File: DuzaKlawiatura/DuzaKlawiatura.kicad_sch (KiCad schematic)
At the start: 29 parts, among them J1 Conn_01x02_Pin, J2 Conn_01x02_Pin, J3 USB_C_Receptacle_USB2.0, U6 STM32F072CBT6, U7 SN74LV1T34DBV, U8 PRTR5V0U2X, U9 XC6206P332MR-Regulator_Linear

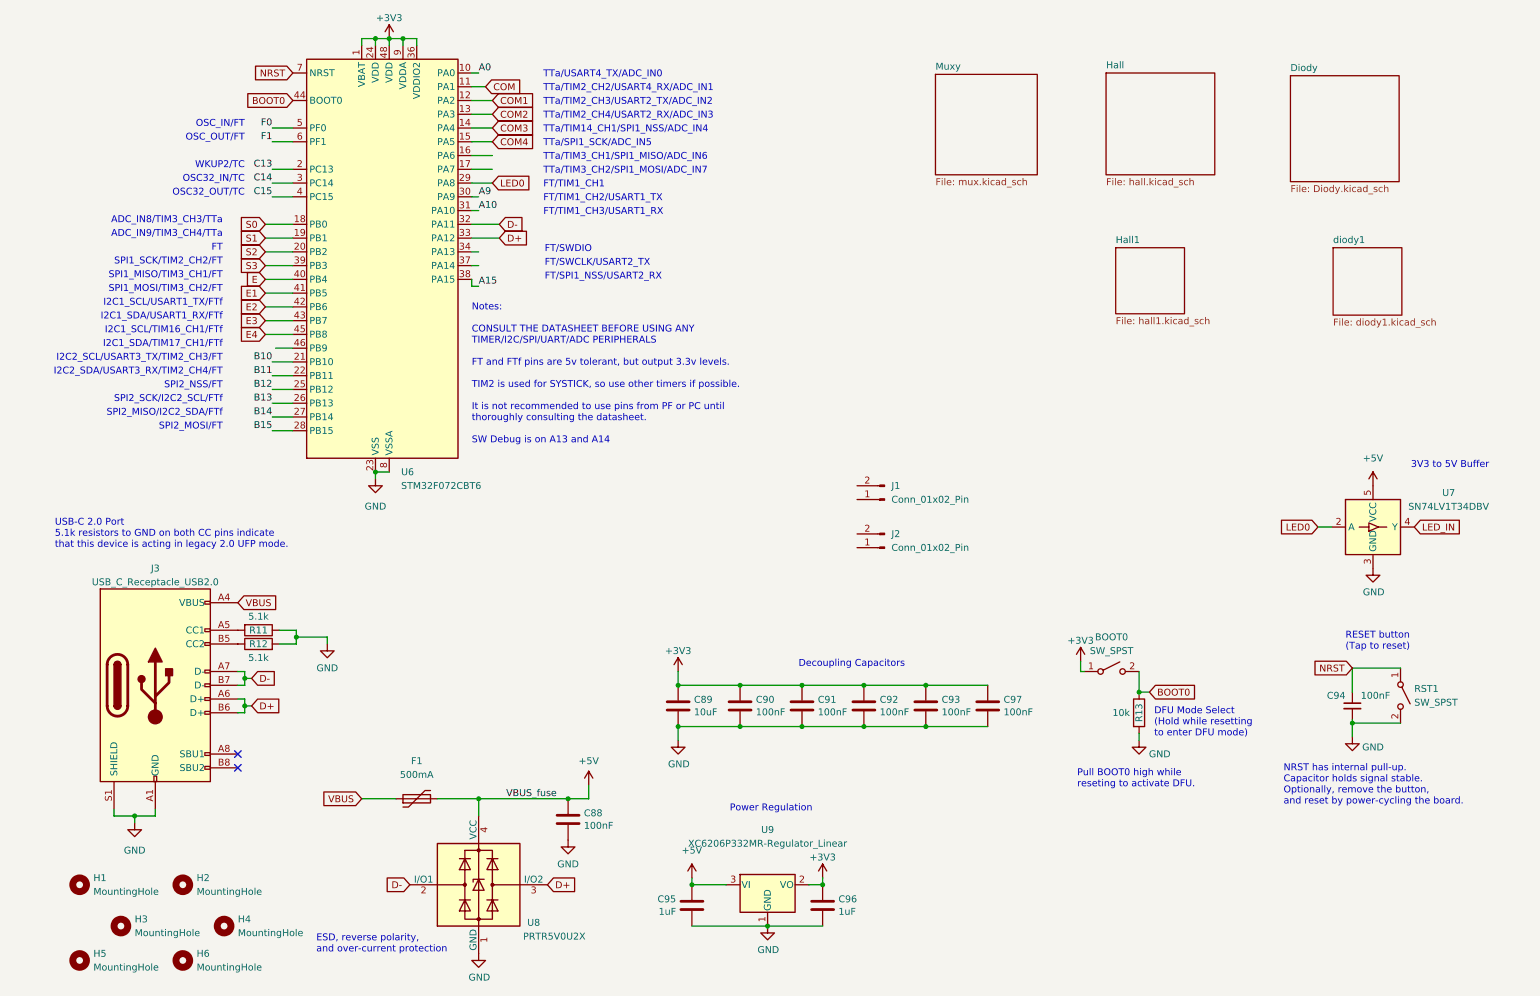
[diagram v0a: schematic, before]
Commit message: Added photos of layout and schematic, updated Kicad files.
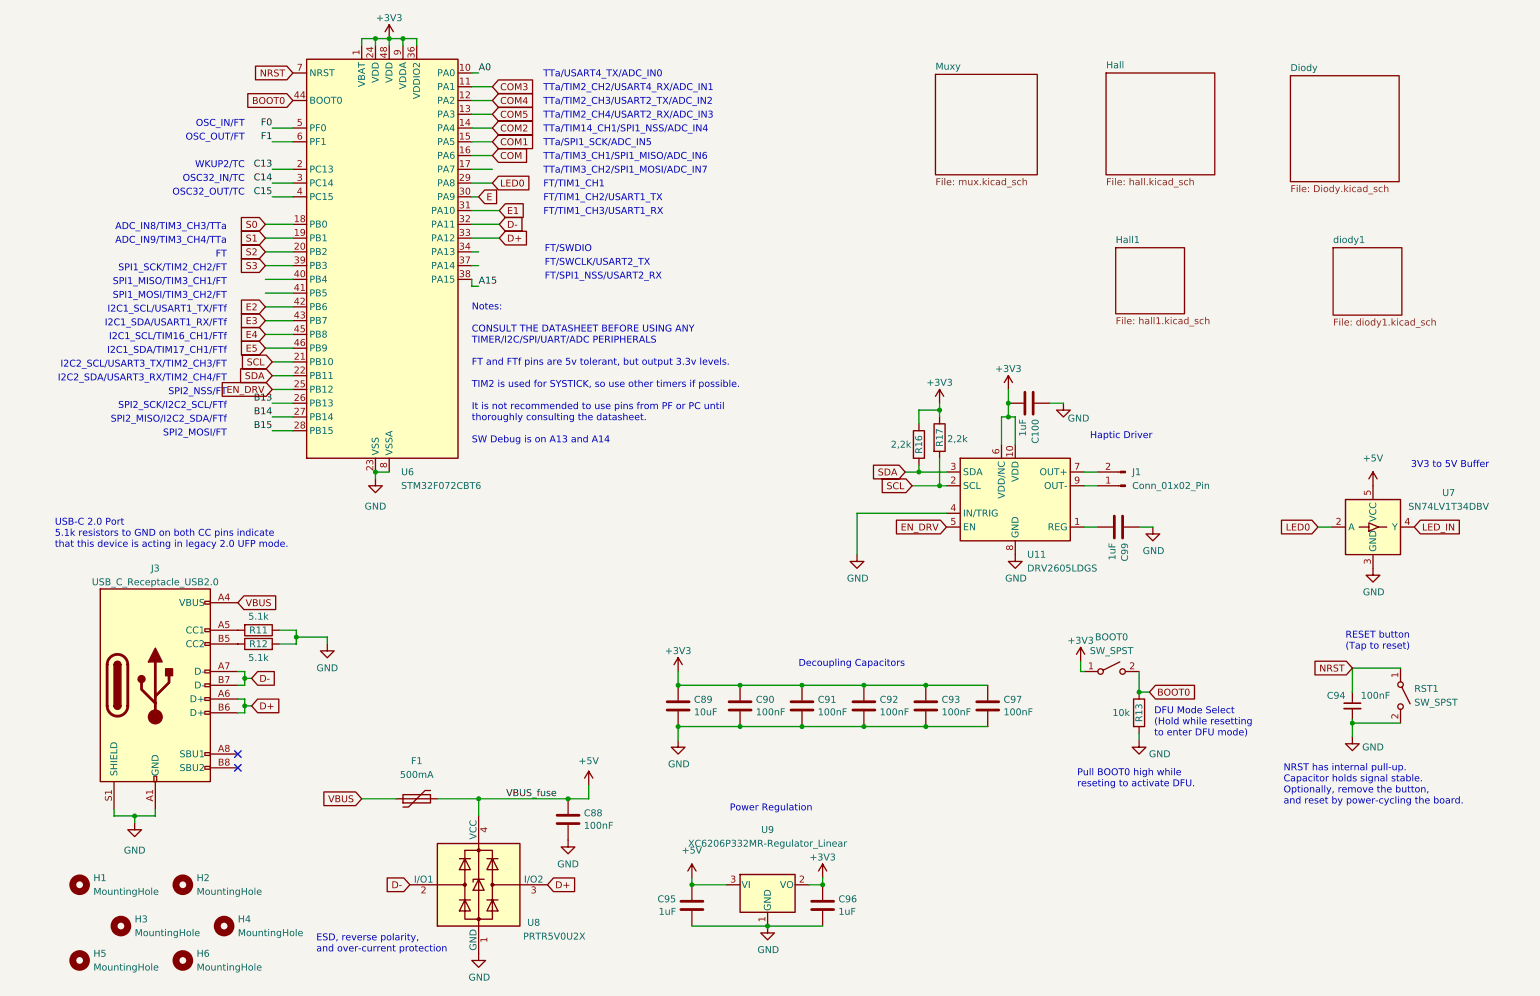
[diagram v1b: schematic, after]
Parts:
- removed J2: Conn_01x02_Pin, MountingHole:MountingHole_2.2mm_M2_ISO7380_Pad, symbol Connector:Conn_01x02_Pin
- added C100, C99: 1uF, Capacitor_SMD:C_0402_1005Metric, symbol Device:C
- added R16, R17: 2,2k, Resistor_SMD:R_0402_1005Metric, symbol Device:R
- added U11: DRV2605LDGS, Package_SO:VSSOP-10_3x3mm_P0.5mm, symbol Driver_Haptic:DRV2605LDGS
- J1: footprint MountingHole:MountingHole_2.2mm_M2_ISO7380_Pad -> Connector_PinHeader_2.54mm:PinHeader_1x02_P2.54mm_Vertical
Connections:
- net A10 is gone; now on net E1: U6.31 (PA10)
- net A9 is gone; now on net E: U6.30 (PA9)
- net +3V3: now also C100.2, R16.1, R17.1, U11.10 (VDD), U11.6 (VDD/NC)
- net COM: now also U6.16 (PA6); no longer U6.11 (PA1)
- net COM1: now also U6.15 (PA5); no longer U6.12 (PA2)
- net COM2: now also U6.14 (PA4); no longer U6.13 (PA3)
- net COM3: now also U6.11 (PA1); no longer U6.14 (PA4)
- net COM4: now also U6.12 (PA2); no longer U6.15 (PA5)
- net E: no longer U6.40 (PB4)
- net E1: no longer U6.41 (PB5)
- net GND: now also C100.1, C99.1, U11.4 (IN/TRIG), U11.8 (GND)
- net at J1.1 (Pin_1): now also U11.9 (OUT-)
- net at J1.2 (Pin_2): now also U11.7 (OUT+)
- net E5: now reaches U6.46 (PB9)
- net B10 renamed SCL
- net SCL: now also R17.2, U11.2 (SCL)
- net B11 renamed SDA
- net SDA: now also R16.2, U11.3 (SDA)
- net B12 renamed EN_DRV
- net EN_DRV: now also U11.5 (EN)
- new net: C99.2, U11.1 (REG)
- new net COM5: U6.13 (PA3)
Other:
- note added: "Haptic Driver"
- moved on the sheet: J1
